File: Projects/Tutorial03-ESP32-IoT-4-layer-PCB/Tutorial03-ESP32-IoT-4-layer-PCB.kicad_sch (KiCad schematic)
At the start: 17 parts, among them J1 SS-52400-002, J2 B2B-PH-SM4-TB, U1 MCP73871

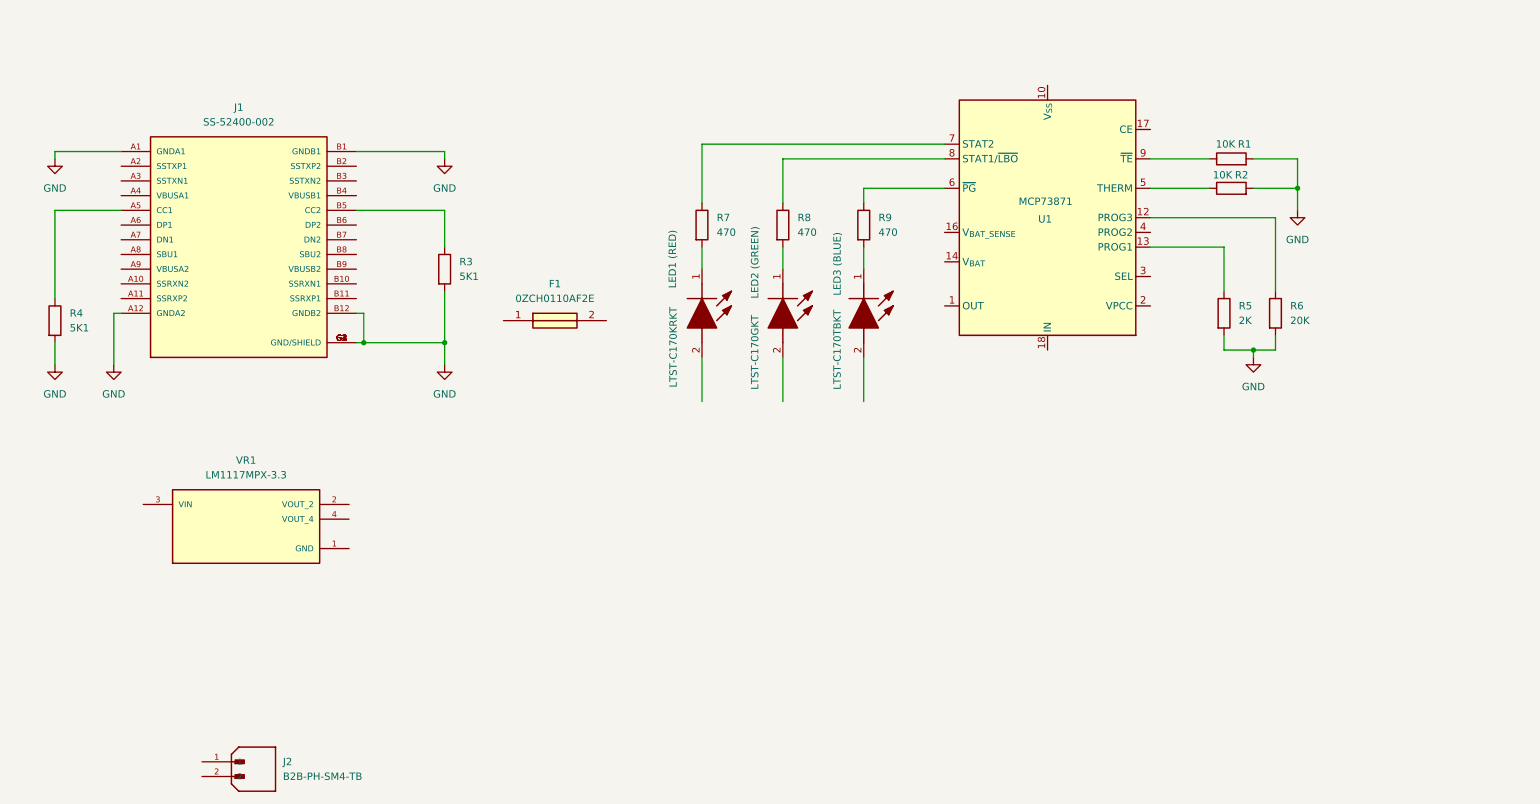
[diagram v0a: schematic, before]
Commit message: 20260207
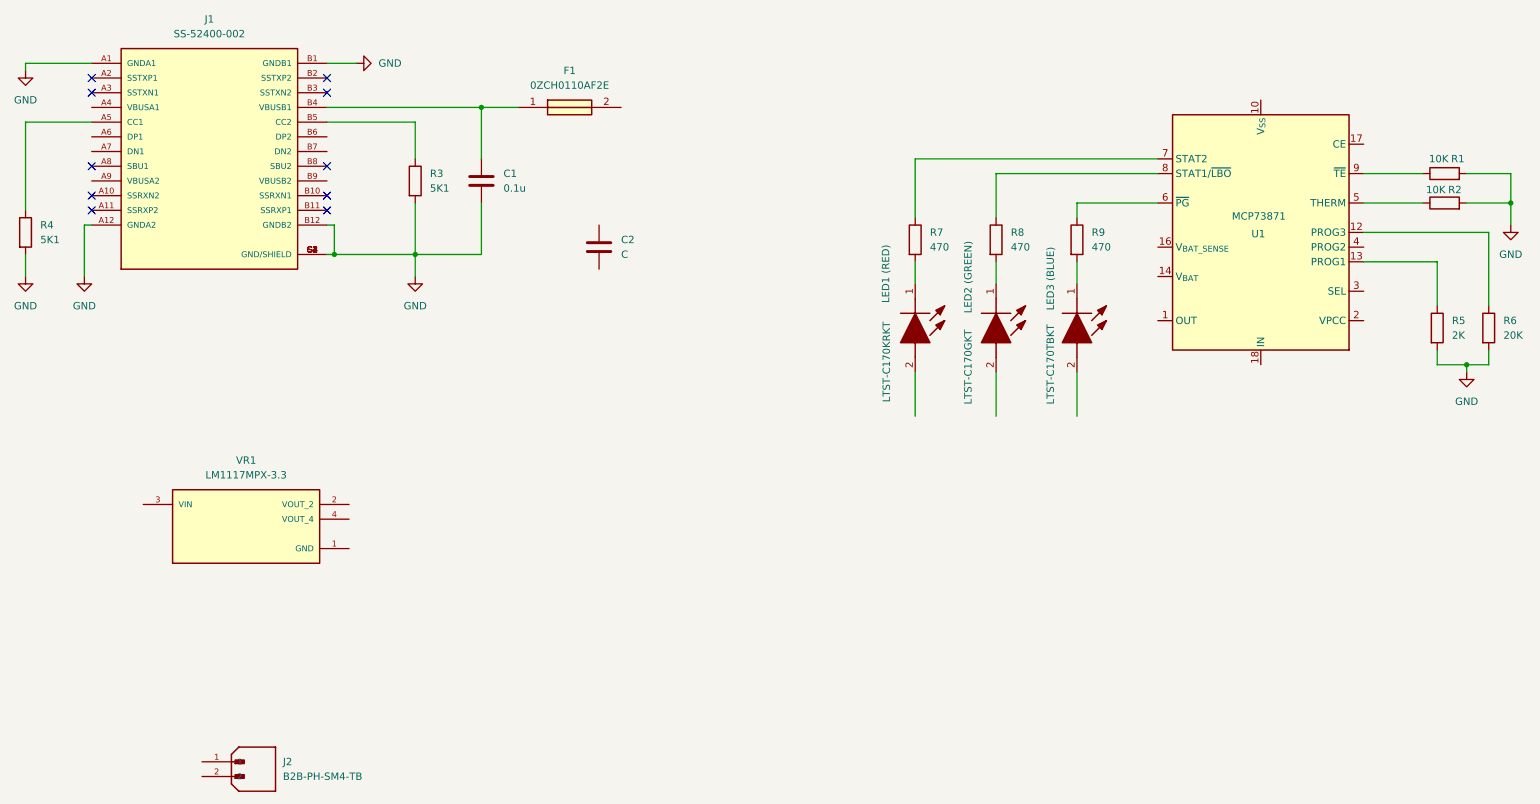
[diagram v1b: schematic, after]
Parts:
- added C1: 0.1u, symbol Device:C
- added C2: C, symbol Device:C
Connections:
- net GND: now also C1.2
- net at J1.B4 (VBUSB1): now also F1.1, C1.1
- no-connect marks 0 -> 10
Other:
- moved on the sheet: F1, J1, LED1 (RED), LED2 (GREEN), LED3 (BLUE), R1, R2, R3, R4, R5, R6, R7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
